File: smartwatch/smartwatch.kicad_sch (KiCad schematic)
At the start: 32 parts, among them J1 BAT_CON, J2 DC_CON, J3 PROG_INT, J4 I2C Touch, J5 SPI Display, J6 Power, J7 Micro_SD_Card, SW1 SW_Push, U1 ESP32-WROVER-E, U2 MCP73831-5-OT, U3 MPU-6050, U3 TLV1117-33

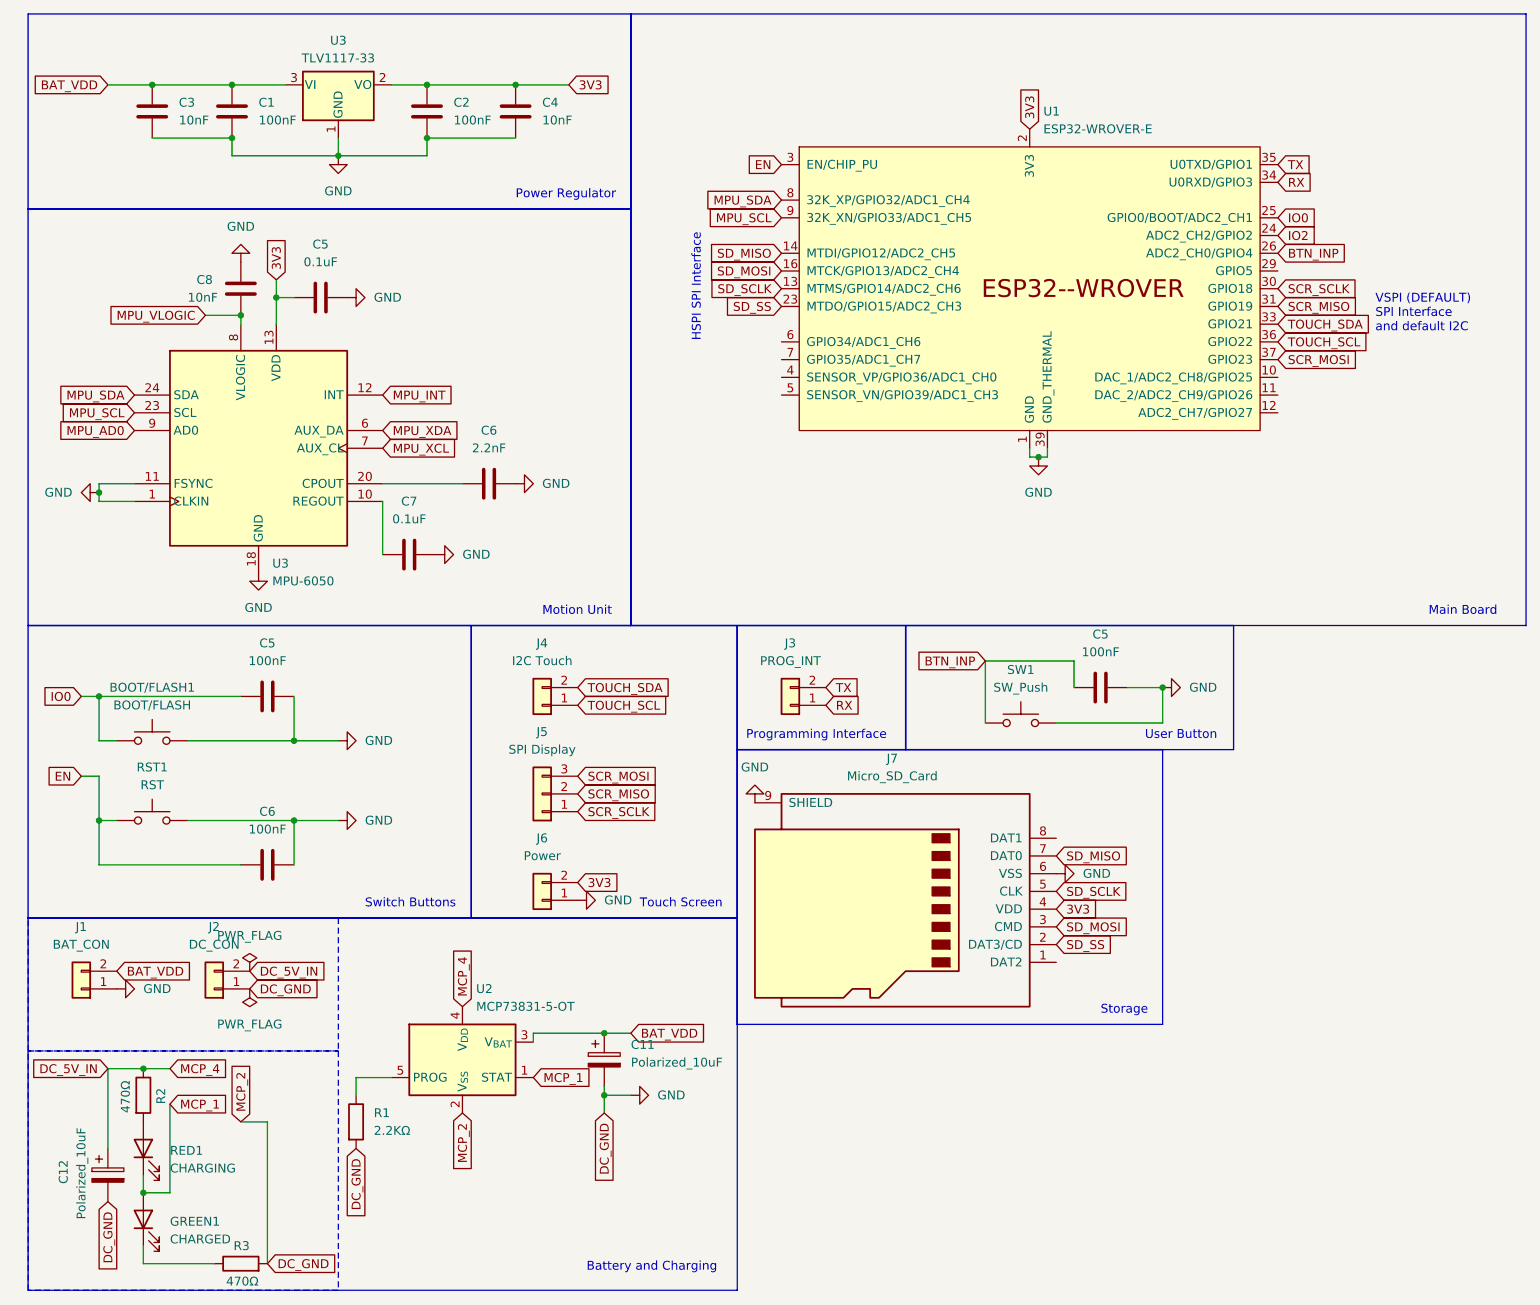
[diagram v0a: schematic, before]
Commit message: updated pcb schematic and design
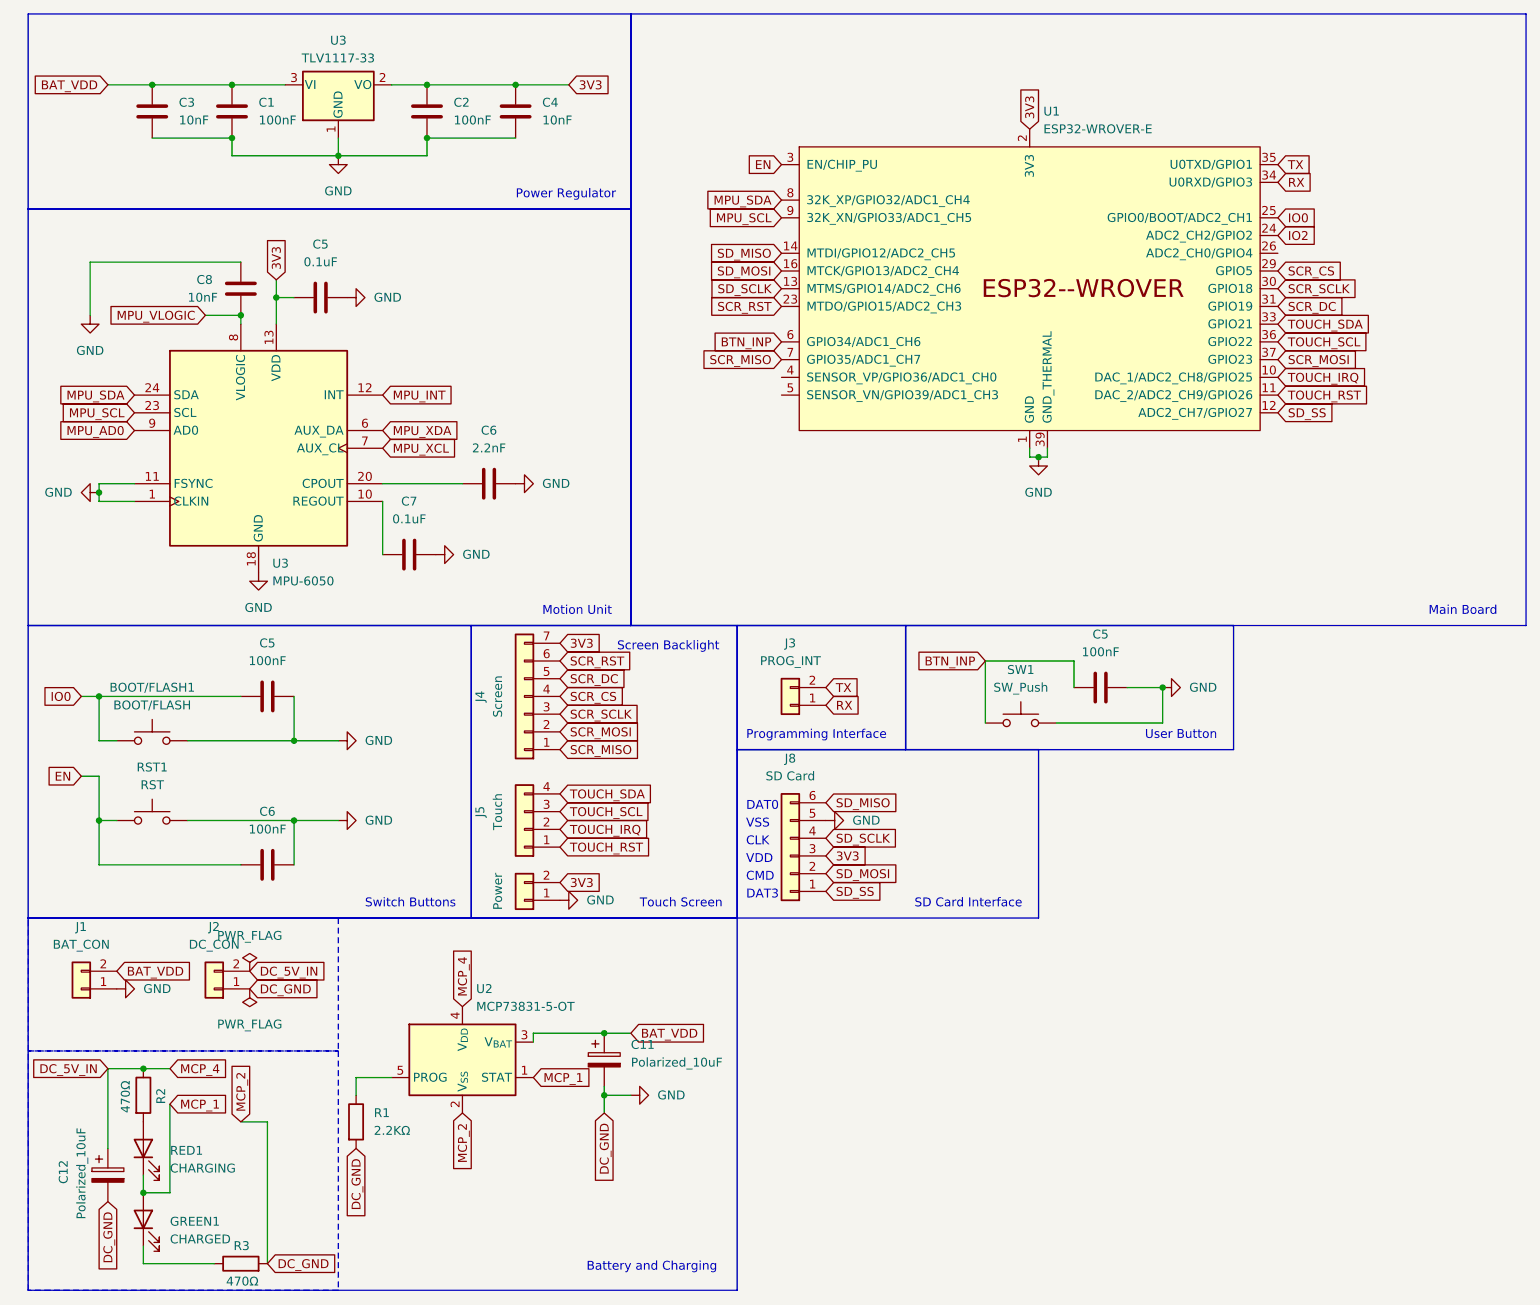
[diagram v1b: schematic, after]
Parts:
- removed J4: I2C Touch, Connector_Wire_SMD:Wire_Pad_1x02, symbol Connector_Generic:Conn_01x02
- removed J5: SPI Display, Connector_Wire_SMD:Wire_Pad_1x03, symbol Connector_Generic:Conn_01x03
- removed J7: Micro_SD_Card, Connector_Card:microSD_HC_Hirose_DM3D-SF, symbol Connector:Micro_SD_Card
- added J4: Screen, Connector_Wire_SMD:Wire_Pad_1x07, symbol Connector_Generic:Conn_01x07
- added J5: Touch, Connector_Wire_SMD:Wire_Pad_1x04, symbol Connector_Generic:Conn_01x04
- added J8: SD Card, Connector_Wire_SMD:Wire_Pad_1x06, symbol Connector_Generic:Conn_01x06
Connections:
- net 3V3: now also J4.7 (Pin_7), J8.3 (Pin_3)
- net BTN_INP: now also U1.6 (GPIO34/ADC1_CH6); no longer U1.26 (ADC2_CH0/GPIO4)
- net GND: now also J8.5 (Pin_5)
- net SCR_MISO: now also U1.7 (GPIO35/ADC1_CH7), J4.1 (Pin_1); no longer U1.31 (GPIO19)
- net SCR_MOSI: now also J4.2 (Pin_2)
- net SCR_SCLK: now also J4.3 (Pin_3)
- net SD_MISO: now also J8.6 (Pin_6)
- net SD_MOSI: now also J8.2 (Pin_2)
- net SD_SCLK: now also J8.4 (Pin_4)
- net SD_SS: now also U1.12 (ADC2_CH7/GPIO27), J8.1 (Pin_1); no longer U1.23 (MTDO/GPIO15/ADC2_CH3)
- net TOUCH_SCL: now also J5.3 (Pin_3)
- net TOUCH_SDA: now also J5.4 (Pin_4)
- net TOUCH_IRQ: now reaches U1.10 (DAC_1/ADC2_CH8/GPIO25)
- net TOUCH_IRQ: now also J5.2 (Pin_2)
- net TOUCH_RST: now reaches U1.11 (DAC_2/ADC2_CH9/GPIO26)
- net TOUCH_RST: now also J5.1 (Pin_1)
- net SCR_CS: now reaches U1.29 (GPIO5)
- net SCR_CS: now also J4.4 (Pin_4)
- new net SCR_DC: J4.5 (Pin_5), U1.31 (GPIO19)
- new net SCR_RST: J4.6 (Pin_6), U1.23 (MTDO/GPIO15/ADC2_CH3)
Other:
- note added: "CLK"
- note added: "CMD"
- note added: "DAT0"
- note added: "DAT3"
- note added: "SD Card Interface"
- note added: "Screen Backlight"
- note added: "VDD"
- note added: "VSS"
- note removed: "HSPI SPI Interface"
- note removed: "Storage"
- note removed: "VSPI (DEFAULT) SPI Interface and default I2C"
- company: (none) -> Xonize Industries
- title: (none) -> Project Zero
